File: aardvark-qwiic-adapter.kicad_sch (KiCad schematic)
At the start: 7 parts, among them J1 Conn_02x05_Odd_Even, J2 Conn_01x04, J3 Conn_01x04, J4 Conn_01x02, U1 AP7361C-33E

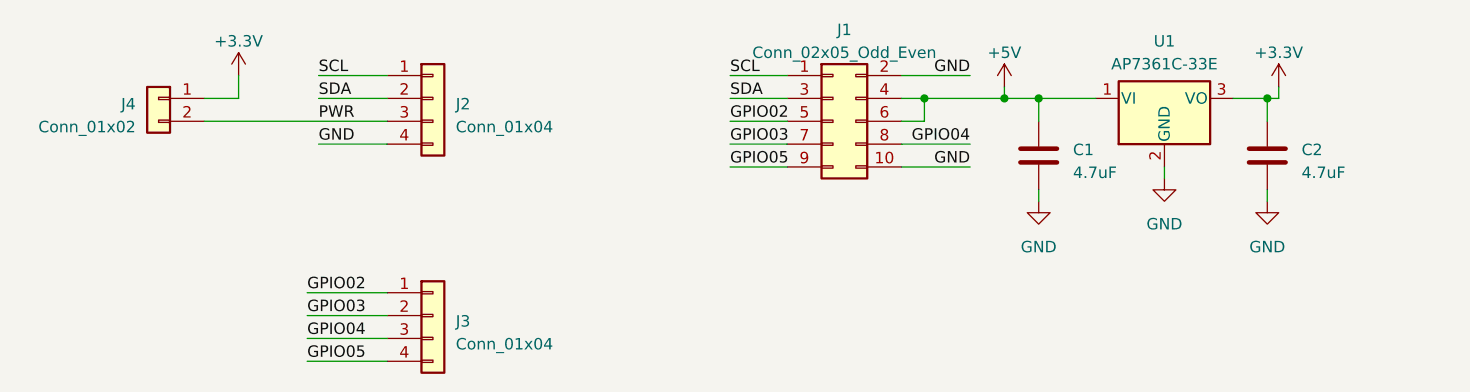
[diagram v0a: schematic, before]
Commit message: ERC
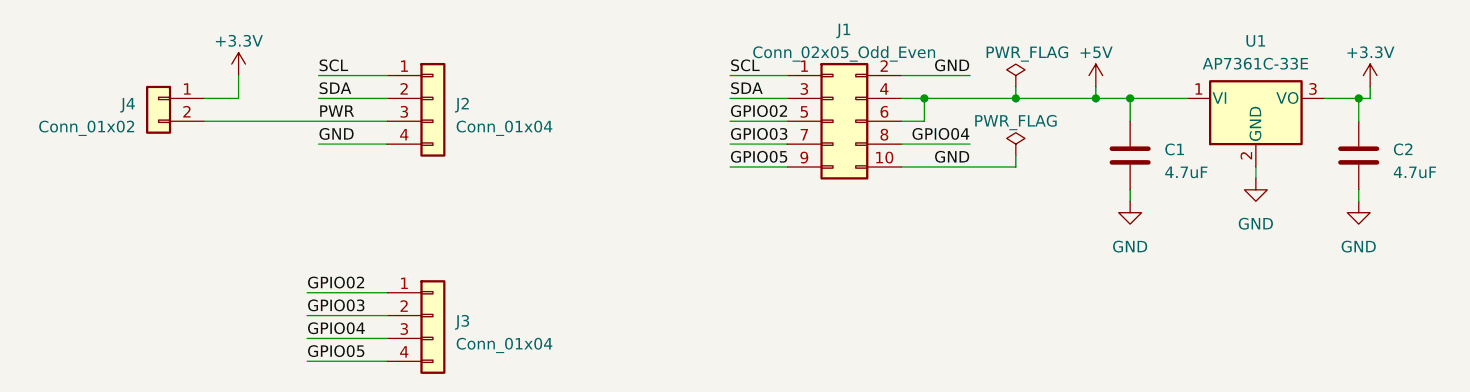
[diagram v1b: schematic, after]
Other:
- moved on the sheet: C1, C2, U1
